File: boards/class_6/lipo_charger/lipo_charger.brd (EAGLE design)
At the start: 11.9 x 31.2 mm, 11 parts, among them IC1 MCP73831/OT

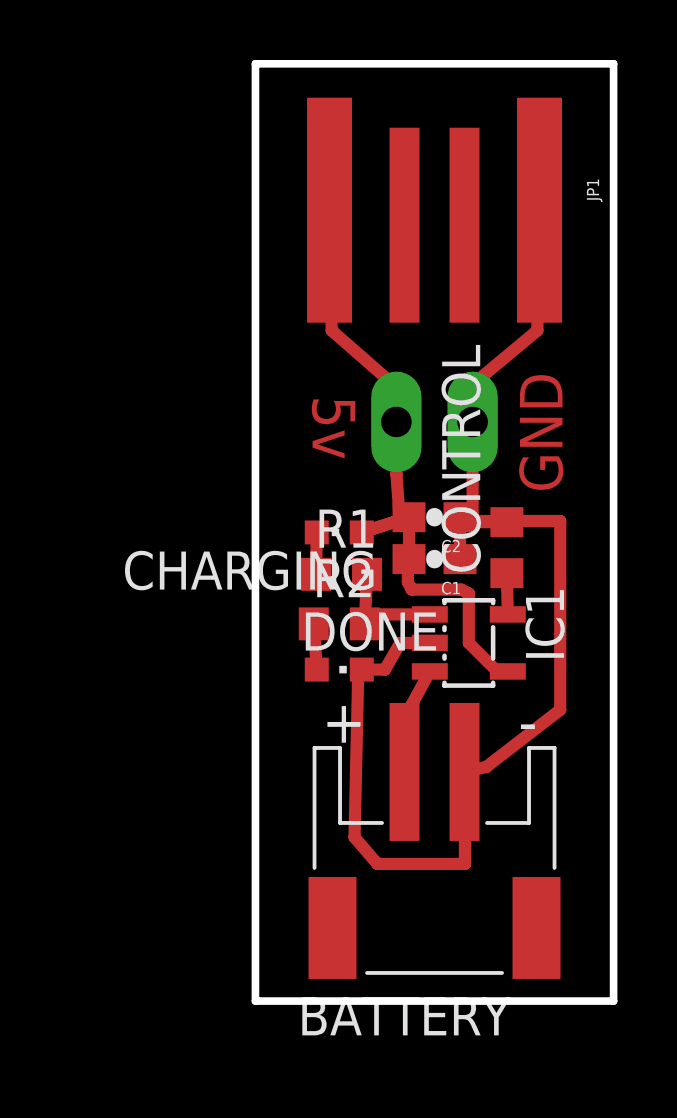
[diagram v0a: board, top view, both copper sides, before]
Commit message: prep lipo board for class 6
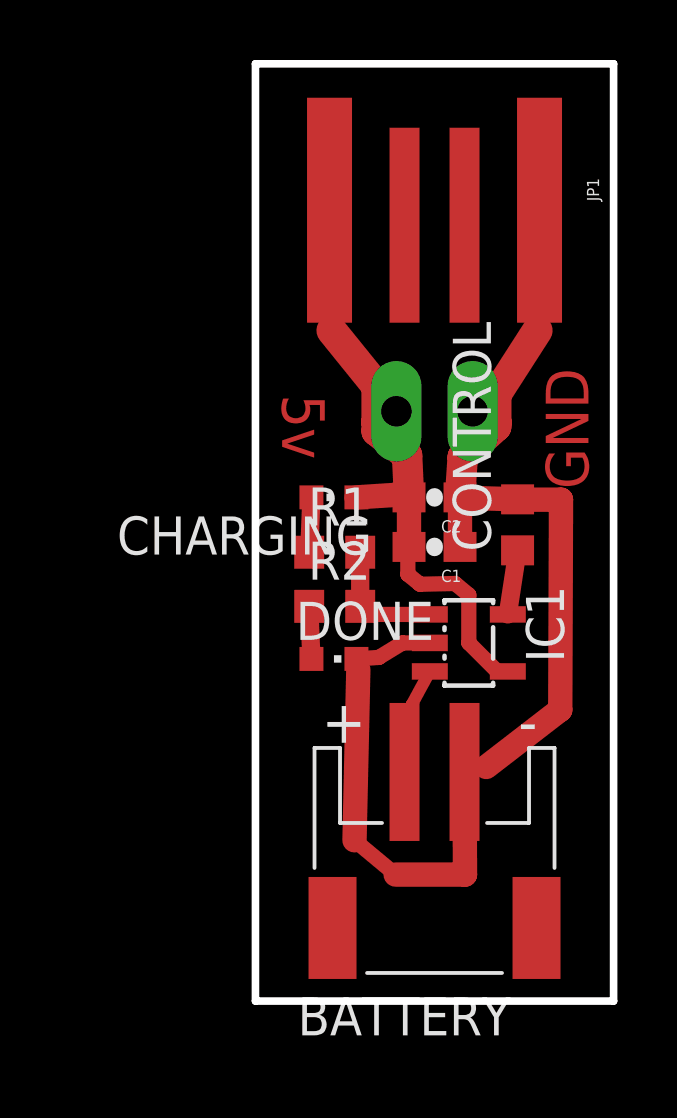
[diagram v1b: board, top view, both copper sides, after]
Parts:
- moved CHARGING 1.18 mm to (6.45, 20.2)
- moved CONTROL 0.84 mm to (12.6, 19.3)
- moved R1 0.77 mm to (6.48, 18.4)
- moved C2 0.66 mm to (9.80, 20.2)
- moved R2 0.60 mm to (6.48, 16.6)
- moved C1 0.41 mm to (9.80, 18.5)
- moved DONE 0.40 mm to (6.45, 14.8)
- moved U$1 0.36 mm to (11.1, 23.1)
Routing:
- net GND: track 43.2 -> 45.4 mm
- net N$6: track 1.38 -> 2.16 mm
